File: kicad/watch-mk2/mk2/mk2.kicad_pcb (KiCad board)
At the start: 2 copper layers, 30 x 60 mm, 71 parts, among them IC1 113990582, IC2 M41T62LC6F, J1 FPC24-0.5mm, J2 USB_C_Receptacle_USB2.0, J3 Conn_01x02_Female, Q1 Si1308EDL, Q2 Si1308EDL, Q3 Si1308EDL, Q4 Si1308EDL, SW1 B5, SW2 B1, SW3 B2, SW4 B3, SW5 B4, U1 W25X20CLUXIG, U2 LM3671MF-2.8_NOPB, U3 MCP73831-2-OT, Y1 32.768kHz

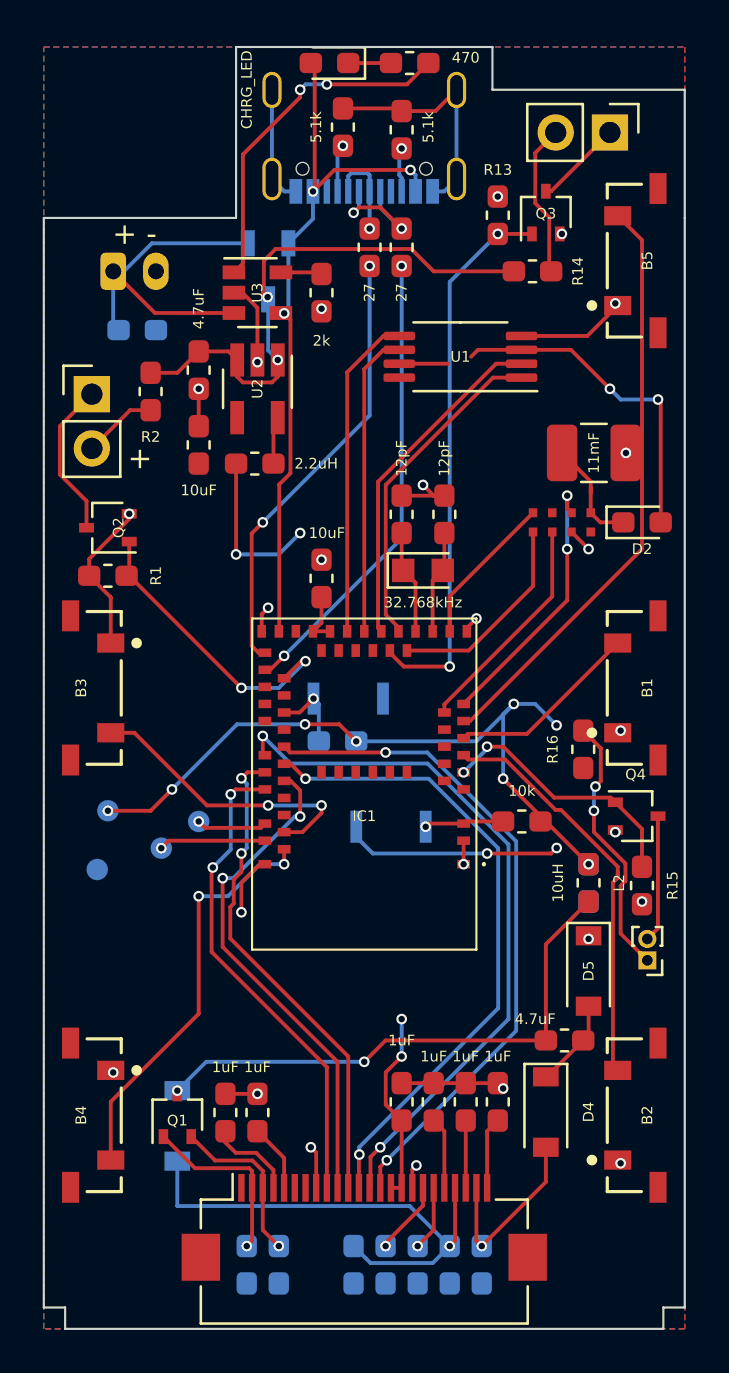
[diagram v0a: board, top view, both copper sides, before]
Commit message: add rev2mk2
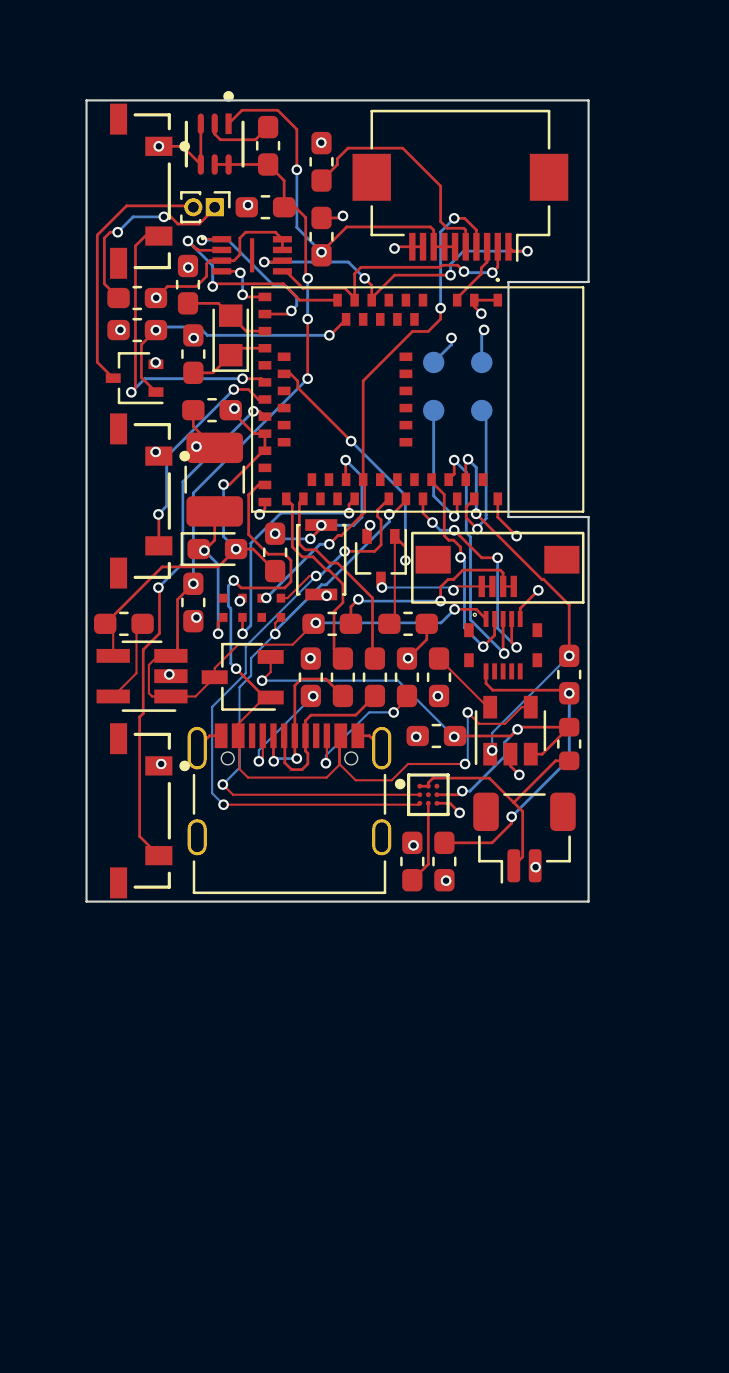
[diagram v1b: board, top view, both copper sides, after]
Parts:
- removed C11, C12, C13, C14, C15, C16, C17, C18, C19: 1uF, Capacitor_SMD:C_0603_1608Metric_Pad1.05x0.95mm_HandSolder
- removed D3, D4, D5: MBR0530, Diode_SMD:D_SOD-123
- removed D6: CHRG_LED, LED_SMD:LED_0603_1608Metric_Pad1.05x0.95mm_HandSolder
- removed D7: FLASHLIGHT, Connector_PinHeader_2.54mm:PinHeader_1x02_P2.54mm_Vertical
- removed D8: BACKLIGHT, Connector_PinHeader_2.54mm:PinHeader_1x02_P2.54mm_Vertical
- removed Q1, Q2: Si1308EDL, Package_TO_SOT_SMD:SOT-323_SC-70
- removed R1, R2: 1k, Resistor_SMD:R_0603_1608Metric_Pad1.05x0.95mm_HandSolder
- removed R10: 470, Resistor_SMD:R_0603_1608Metric_Pad1.05x0.95mm_HandSolder
- removed R7: 10k, Resistor_SMD:R_0603_1608Metric_Pad1.05x0.95mm_HandSolder
- removed R8: 3, Resistor_SMD:R_0603_1608Metric_Pad1.05x0.95mm_HandSolder
- removed SW3: B2, libs:E-Switch-TL3330AF130QG-MFG
- removed SW5: B4, libs:E-Switch-TL3330AF130QG-MFG
- removed SW_BOOT1: SW_Push, Button_Switch_SMD:SW_SPST_CK_KXT3
- added J5: Conn_01x04_Female, libs:ffc-0.5mm-4, F.Cu at (31.2, 35.2)
- added JP1: FUEL_BYP, Resistor_SMD:R_0603_1608Metric, F.Cu at (34.6, 42.6)
- added P1: AXT610124, libs:PANASONIC_AXT610124, F.Cu at (31.5, 38.0)
- added U5: MAX17220ELT+, max17220:Maxim_Integrated-L622-1C-0-E-IPC_A, F.Cu at (18.0, 14.5)
- added U6: MAX17262REWL+T, max17262:Maxim-W91G1-3-0-A-IPC_A, F.Cu at (28.0, 45.0)
- BT1: footprint Connector_JST:JST_PH_B2B-PH-K_1x02_P2.00mm_Vertical -> Connector_JST:JST_SH_BM02B-SRSS-TB_1x02-1MP_P1.00mm_Vertical; moved to F.Cu
- C10: value 1uF -> 0.47uF; moved to F.Cu
- C20, D1, J2, R6, SW_RESET1: moved to F.Cu
- C6: value 4.7uF -> 10uF; moved to F.Cu
- C8: value 4.7uF -> 10uF
- C9: value 1uF -> 560pF; moved to F.Cu
- IC1: value 113990582 -> MDBT50Q
- J1: value FPC24-0.5mm -> Conn_01x10_Female; footprint Connector_FFC-FPC:Hirose_FH12-24S-0.5SH_1x24-1MP_P0.50mm_Horizontal -> Connector_FFC-FPC:Hirose_FH12-10S-0.5SH_1x10-1MP_P0.50mm_Horizontal
- L2: value 10uH -> 2.2uH
- R13, R15: value 1k -> 100k
- R5: value 10k -> 100k
- U1: footprint Package_SO:TSSOP-8_4.4x3mm_P0.65mm -> libs:SON50P300X200X60-9N
- moved C9 51.6 mm to (23.0, 15.4), turned to 90 degrees
- moved J1 48.0 mm to (29.5, 17.5), turned to 180 degrees
- moved J3 40.7 mm to (18.0, 17.5), turned to -90 degrees
- moved C8 39.3 mm to (23.0, 18.9), turned to 90 degrees
- moved L2 37.6 mm to (20.5, 14.6), turned to 90 degrees
- moved R15 35.1 mm to (14.4, 23.2), turned to 180 degrees
- moved C6 35.1 mm to (20.4, 17.5), turned to 180 degrees
- moved SW2 33.6 mm to (14.0, 16.8), turned to -90 degrees
- moved BT1 32.8 mm to (32.5, 47.0)
- moved Q4 31.2 mm to (14.2, 25.5), turned to 180 degrees
- moved J2 30.7 mm to (21.5, 44.8)
- moved R16 29.7 mm to (14.4, 21.8), turned to 180 degrees
- moved TP3 27.3 mm to (30.5, 24.8), turned to 180 degrees
- moved SW1 26.7 mm to (14.0, 31.2), turned to -90 degrees
- moved TP4 26.6 mm to (28.2, 27.0), turned to 180 degrees
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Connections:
- C10 pad 1: GND -> Net-(C10-Pad1)
- C10 pad 2: /EPVPP -> GND
- C20 pad 1: +BATT -> BATTPOW
- C6 pad 1: GND -> VIN
- C6 pad 2: VCC -> GND
- C8 pad 1: Net-(C8-Pad1) -> 5V
- C8 pad 2: Net-(C8-Pad2) -> GND
- C9 pad 1: /EPPREVGH -> LCD_DISP
- D1 pad 1: +BATT -> VUSB
- D1 pad 2: VUSB -> BATTPOW
- IC1 pad 10: BUTTON1 -> SPI_CLK
- IC1 pad 12: BUTTON5 -> SPI_MOSI
- IC1 pad 13: SQW -> BUZZER
- IC1 pad 14: RTCIRQ -> SPI_MISO
- IC1 pad 16: SCL -> FLASH_CS
- IC1 pad 19: SDA -> (no net)
- IC1 pad 20: FLASH_CS -> (no net)
- IC1 pad 22: FLASH_DO -> BUTTON1
- IC1 pad 24: FLASH_CLK -> BUTTON5
- IC1 pad 26: FLASH_DI -> BUTTON3
- IC1 pad 3: BOOTLOAD -> LCD_CS
- IC1 pad 36: FLASHLIGHT -> (no net)
- IC1 pad 41: (no net) -> RTCIRQ
- IC1 pad 42: (no net) -> SQW
- IC1 pad 43: EPSDIN -> (no net)
- IC1 pad 44: EPSCLK -> SDA
- IC1 pad 45: EPCS -> (no net)
- IC1 pad 46: EPDC -> SCL
- IC1 pad 47: EPRES -> (no net)
- IC1 pad 48: EPBUSY -> BUTTON4
- IC1 pad 49: (no net) -> FLASHLIGHT
- IC1 pad 50: (no net) -> BUTTON2
- IC1 pad 52: BUTTON3 -> CHGNG
- IC1 pad 54: BUTTON4 -> (no net)
- IC1 pad 6: BUZZER -> (no net)
- IC1 pad 8: BUTTON2 -> (no net)
- J1 pad 1: (no net) -> SPI_CLK
- J1 pad 10: EPRES -> GND
- J1 pad 2: /EPGDR -> SPI_MOSI
- J1 pad 3: /EPRESE -> LCD_CS
- J1 pad 4: /EPVGL -> SQW
- J1 pad 5: /EPVGH -> LCD_DISP
- J1 pad 6: (no net) -> 5V
- J1 pad 7: (no net) -> 5V
- J1 pad 8: GND -> 5V
- J1 pad 9: EPBUSY -> GND
- L2 pad 1: VCC -> VIN
- L2 pad 2: Net-(C8-Pad1) -> Net-(L2-Pad2)
- R5 pad 1: VCC -> CHGNG
- R5 pad 2: BOOTLOAD -> VCC
- TP1 pad 1: SWDIO -> GND
- TP4 pad 1: GND -> SWDIO
- U1 pad 2: FLASH_DO -> SPI_MISO
- U1 pad 5: FLASH_DI -> SPI_MOSI
- U1 pad 6: FLASH_CLK -> SPI_CLK
- U3 pad 1: Net-(R10-Pad1) -> CHGNG
- U3 pad 3: +BATT -> BATTPOW
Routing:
- net GND: track 66.2 -> 30.5 mm, vias 27 -> 33
- net EPSCLK: track 33.3 -> 0.00 mm, vias 2 -> 0
- net EPSDIN: track 31.5 -> 0.00 mm, vias 2 -> 0
- net EPCS: track 30.3 -> 0.00 mm, vias 2 -> 0
- net Net-(C8-Pad1): track 25.9 -> 0.00 mm, vias 2 -> 0
- net VCC: track 71.1 -> 46.0 mm, vias 14 -> 7
- net BATTPOW: track 0.00 -> 24.7 mm, vias 0 -> 4
- net VIN: track 25.5 -> 49.7 mm, vias 2 -> 6
- net EPRES: track 23.7 -> 0.00 mm, vias 2 -> 0
- net /EPPREVGH: track 23.6 -> 0.00 mm, vias 1 -> 0
- net EPDC: track 23.1 -> 0.00 mm, vias 2 -> 0
- net EPBUSY: track 22.7 -> 0.00 mm, vias 2 -> 0
- net SDA: track 9.68 -> 30.3 mm, vias 0 -> 3
- net SCL: track 7.17 -> 27.5 mm, vias 0 -> 3
- net CHGNG: track 0.00 -> 18.3 mm, vias 0 -> 4
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- added copper zone on In2.Cu, net GND
- added copper zone on In1.Cu, net VCC
- removed copper zone on B.Cu, net GND
- removed copper zone on F.Cu, net VCC
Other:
- board size 30 x 60 mm -> 23.5 x 37.5 mm
- copper layers 2 -> 4
- board text added: "+2.8v"
- board text added: "nrf52-watch mk2 - rev.2"
- board text removed: "+"
- board text removed: "+ -"
- board text removed: "+2.8V"
- board text removed: "-"
- board text removed: "Backlight"
- board text removed: "Flashlight"
- board text removed: "buzzer"
- board text removed: "nrf52-watch mk2 - rev.1"
